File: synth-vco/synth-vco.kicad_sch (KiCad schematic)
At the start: 146 parts, among them J1 Conn_Coaxial, J2 Screw_Terminal_01x10, J3 Screw_Terminal_01x05, J4 Conn_Coaxial, J5 Barrel_Jack, U1 ADF4158, U10 LT3045IMSE_TRPBF, U11 LT3045IMSE_TRPBF, U12 LT3045IMSE_TRPBF, U13 LT8570EMS8E_TRPBF, U14 LT3065EDDPBF, U15 LT3065EDDPBF, U16 BT09E, U3 ADP-2-10+, U4 DAT-15R5A-SP+, U5 OPA192IDGKT, U6 TPSM53602RDAR, U7 LT3045IMSE_TRPBF, U8 LT3045IMSE_TRPBF, U9 LT3045IMSE_TRPBF, Y3 CVCO55CW-0500-1000

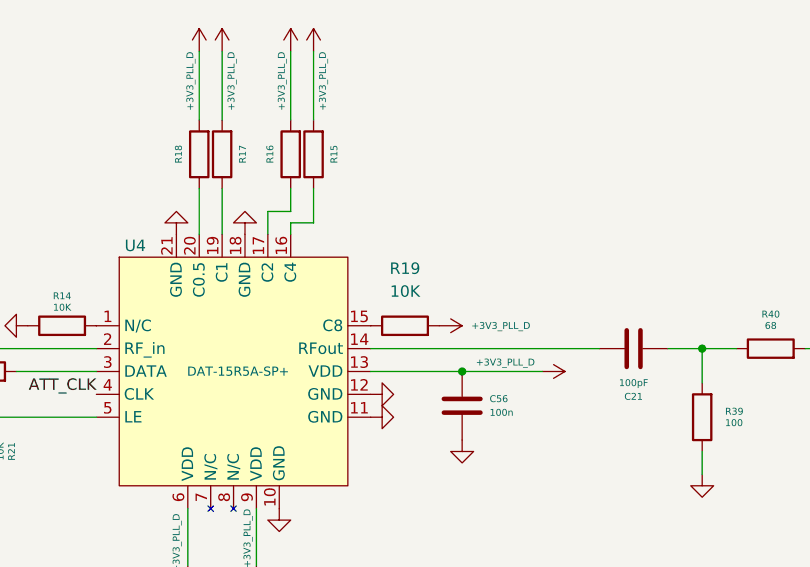
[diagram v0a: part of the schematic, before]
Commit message: fix: resistors, capacitors and inductors footprints
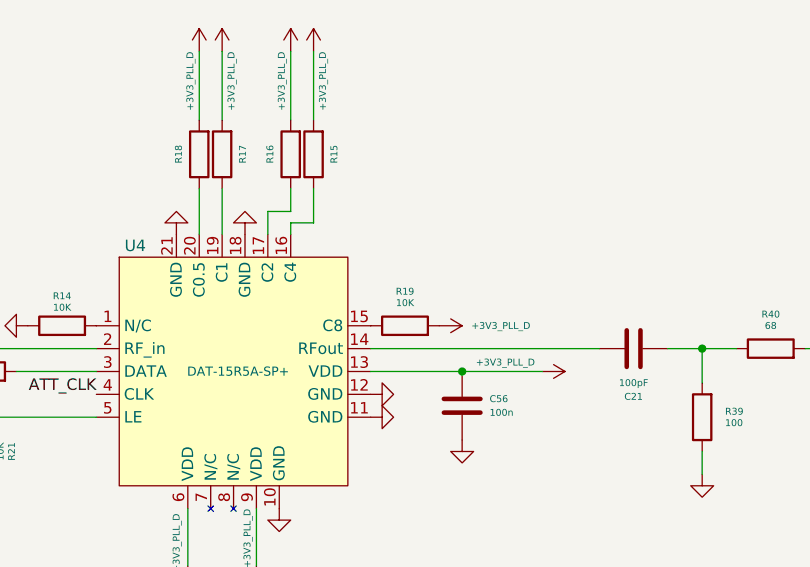
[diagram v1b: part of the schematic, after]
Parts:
- C1, C12, C13, C14, C15, C16, C17, C2, C20, C21, C22, C4, C5, C66, C67, C68, C69, C71, C72: footprint (none) -> Capacitor_SMD:C_0603_1608Metric_Pad1.08x0.95mm_HandSolder
- C23, C24, C29, C30, C31, C32, C33, C34, C35, C36, C38, C39, C41, C42, C44: footprint Capacitor_SMD:C_0603_1608Metric_Pad1.08x0.95mm_HandSolder -> Capacitor_SMD:C_0805_2012Metric_Pad1.18x1.45mm_HandSolder
- C25, C26, C27, C28, C49, C51, C55, C65: footprint Capacitor_SMD:C_0603_1608Metric_Pad1.08x0.95mm_HandSolder -> Capacitor_SMD:C_1206_3216Metric_Pad1.33x1.80mm_HandSolder
- C56: footprint Capacitor_SMD:C_0201_0603Metric_Pad0.64x0.40mm_HandSolder -> Capacitor_SMD:C_0603_1608Metric_Pad1.08x0.95mm_HandSolder
- C6, C7: footprint Capacitor_SMD:C_0201_0603Metric_Pad0.64x0.40mm_HandSolder -> Capacitor_SMD:C_1206_3216Metric_Pad1.33x1.80mm_HandSolder
- C70: footprint (none) -> Capacitor_SMD:C_0805_2012Metric_Pad1.18x1.45mm_HandSolder
- C9: footprint (none) -> Capacitor_SMD:C_1206_3216Metric_Pad1.33x1.80mm_HandSolder
- L1, L3, L4, L5, L6: footprint Inductor_SMD:L_0201_0603Metric_Pad0.64x0.40mm_HandSolder -> Inductor_SMD:L_0603_1608Metric_Pad1.05x0.95mm_HandSolder
- R1, R2, R22, R23, R24, R25, R26, R27, R28, R29, R30, R31, R32, R33, R34, R35, R36, R37, R38, R4: footprint Resistor_SMD:R_0201_0603Metric_Pad0.64x0.40mm_HandSolder -> Resistor_SMD:R_0603_1608Metric_Pad0.98x0.95mm_HandSolder
- R10, R11, R12, R13, R14, R15, R16, R17, R18, R19, R20, R21, R3, R39, R40, R41, R5, R6, R8, R9: footprint Resistor_SMD:R_01005_0402Metric_Pad0.57x0.30mm_HandSolder -> Resistor_SMD:R_0603_1608Metric_Pad0.98x0.95mm_HandSolder
- R7: footprint (none) -> Resistor_SMD:R_0603_1608Metric_Pad0.98x0.95mm_HandSolder
